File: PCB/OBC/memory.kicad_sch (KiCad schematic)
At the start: 14 parts, among them U10 TMUX1574PWR, U11 W25Q128JVSIQ, U12 TMUX1574PWR, U9 W25Q128JVSIQ

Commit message: Cambio de OCP
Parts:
- U10, U12: LCSC Part Name (none) -> C2673443
- U11, U9: LCSC Part Name (none) -> C97521

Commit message: Bom resistors
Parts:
- C53, C54, C56, C58: LCSC Part Name (none) -> C1711
- R16, R17, R18, R19: LCSC Part Name (none) -> C2907219
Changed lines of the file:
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@@
+			)
+		)
+		(property "LCSC Part Name" "C2907219"
+			(at 254 80.01 0)
+			(effects
+				(font
+					(size 1.27 1.27)
+				)
+				(hide yes)
 			)
 		)
@@
 		)
 		(property "Mouser" ""
+			(at 129.54 72.39 0)
+			(effects
+				(font
+					(size 1.27 1.27)
+				)
+				(hide yes)
+			)
+		)
+		(property "LCSC Part Name" "C1711"
 			(at 129.54 72.39 0)
 			(effects
@@
 			)
 		)
+		(property "LCSC Part Name" "C1711"
+			(at 269.24 127 0)
+			(effects
+				(font
+					(size 1.27 1.27)
+				)
+				(hide yes)
+			)
+		)
 		(pin "2"
 		)
@@
 			)
 		)
+		(property "LCSC Part Name" "C1711"
+			(at 199.39 62.23 0)
+			(effects
+				(font
+					(size 1.27 1.27)
+				)
+				(hide yes)
+			)
+		)
 		(pin "1"
 		)
@@
 			)
 		)
+		(property "LCSC Part Name" "C2907219"
+			(at 34.29 74.93 90)
+			(effects
+				(font
+					(size 1.27 1.27)
+				)
+				(hide yes)
+			)
+		)
 		(pin "2"
 		)
@@
 			)
 		)
+		(property "LCSC Part Name" "C2907219"
+			(at 109.22 67.31 0)
+			(effects
+				(font
+					(size 1.27 1.27)
+				)
+				(hide yes)
+			)
+		)
 		(pin "1"
 		)
@@
 			)
 		)
+		(property "LCSC Part Name" "C1711"
+			(at 119.38 116.84 0)
+			(effects
+				(font
+					(size 1.27 1.27)
+				)
+				(hide yes)
+			)
+		)
 		(pin "2"
 		)
@@
 			(at 173.99 88.9 90)
 			(effects
+				(font
+					(size 1.27 1.27)
+				)
+				(hide yes)
+			)
+		)
+		(property "LCSC Part Name" "C2907219"
+			(at 173.99 88.9 90)
+			(effects

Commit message: BOM terminado
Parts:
- C53, C54, C56, C58, U10, U11, U12, U9: now left out of the parts list
- C55: footprint XTAL_NX3215SA_NDK:XTAL_NX3215SA_NDK -> Capacitor_SMD:C_0805_2012Metric_Pad1.18x1.45mm_HandSolder; LCSC Part Name (none) -> C28323; now left out of the parts list
- C57: footprint TMUX1574PWR:PWP16_2P31X2P46_TEX -> Capacitor_SMD:C_0805_2012Metric_Pad1.18x1.45mm_HandSolder; LCSC Part Name (none) -> C28323; now left out of the parts list
- R16, R17, R18, R19: footprint (none) -> Resistor_SMD:R_0805_2012Metric_Pad1.20x1.40mm_HandSolder; now left out of the parts list
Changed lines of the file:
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@@
 		(unit 1)
 		(exclude_from_sim no)
-		(in_bom yes)
+		(in_bom no)
 		(on_board yes)
 		(dnp no)
@@
 			)
 		)
-		(property "Footprint" ""
+		(property "Footprint" "Resistor_SMD:R_0805_2012Metric_Pad1.20x1.40mm_HandSolder"
 			(at 252.222 80.01 90)
 			(effects
@@
 		(unit 1)
 		(exclude_from_sim no)
-		(in_bom yes)
+		(in_bom no)
 		(on_board yes)
 		(dnp no)
@@
 			)
 		)
-		(property "Footprint" "TMUX1574PWR:PWP16_2P31X2P46_TEX"
+		(property "Footprint" "Capacitor_SMD:C_0805_2012Metric_Pad1.18x1.45mm_HandSolder"
 			(at 213.0552 66.04 0)
 			(effects
@@
 			)
 		)
+		(property "LCSC Part Name" "C28323"
+			(at 212.09 62.23 0)
+			(effects
+				(font
+					(size 1.27 1.27)
+				)
+				(hide yes)
+			)
+		)
 		(pin "1"
 		)
@@
 		(unit 1)
 		(exclude_from_sim no)
-		(in_bom yes)
+		(in_bom no)
 		(on_board yes)
 		(dnp no)
@@
 			)
 		)
-		(property "Footprint" "XTAL_NX3215SA_NDK:XTAL_NX3215SA_NDK"
+		(property "Footprint" "Capacitor_SMD:C_0805_2012Metric_Pad1.18x1.45mm_HandSolder"
 			(at 143.2052 76.2 0)
 			(effects
@@
 			)
 		)
+		(property "LCSC Part Name" "C28323"
+			(at 142.24 72.39 0)
+			(effects
+				(font
+					(size 1.27 1.27)
+				)
+				(hide yes)
+			)
+		)
 		(pin "1"
 		)
@@
 		(unit 1)
 		(exclude_from_sim no)
-		(in_bom yes)
+		(in_bom no)
 		(on_board yes)
 		(dnp no)
@@
 		(unit 1)
 		(exclude_from_sim no)
-		(in_bom yes)
+		(in_bom no)
 		(on_board yes)
 		(dnp no)
@@
 		(unit 1)
 		(exclude_from_sim no)
-		(in_bom yes)
+		(in_bom no)
 		(on_board yes)
 		(dnp no)
@@
 		(unit 1)
 		(exclude_from_sim no)
-		(in_bom yes)
+		(in_bom no)
 		(on_board yes)
 		(dnp no)
@@
 		(unit 1)
 		(exclude_from_sim no)
-		(in_bom yes)
+		(in_bom no)
 		(on_board yes)
 		(dnp no)
@@
 			)
 		)
-		(property "Footprint" ""
+		(property "Footprint" "Resistor_SMD:R_0805_2012Metric_Pad1.20x1.40mm_HandSolder"
 			(at 34.29 73.152 90)
 			(effects
@@
 		(unit 1)
 		(exclude_from_sim no)
-		(in_bom yes)
+		(in_bom no)
 		(on_board yes)
 		(dnp no)
@@
 			)
 		)
-		(property "Footprint" ""
+		(property "Footprint" "Resistor_SMD:R_0805_2012Metric_Pad1.20x1.40mm_HandSolder"
 			(at 107.442 67.31 90)
 			(effects
@@
 		(unit 1)
 		(exclude_from_sim no)
-		(in_bom yes)
+		(in_bom no)
 		(on_board yes)
 		(dnp no)
@@
 		(unit 1)
 		(exclude_from_sim no)
-		(in_bom yes)
+		(in_bom no)
 		(on_board yes)
 		(dnp no)
@@
 		(unit 1)
 		(exclude_from_sim no)
-		(in_bom yes)
+		(in_bom no)
 		(on_board yes)
 		(dnp no)
@@
 			)
 		)
-		(property "Footprint" ""
+		(property "Footprint" "Resistor_SMD:R_0805_2012Metric_Pad1.20x1.40mm_HandSolder"
 			(at 173.99 87.122 90)
 			(effects
@@
 		(unit 1)
 		(exclude_from_sim no)
-		(in_bom yes)
+		(in_bom no)
 		(on_board yes)
 		(dnp no)
@@
 		(unit 1)
 		(exclude_from_sim no)
-		(in_bom yes)
+		(in_bom no)
 		(on_board yes)
 		(dnp no)

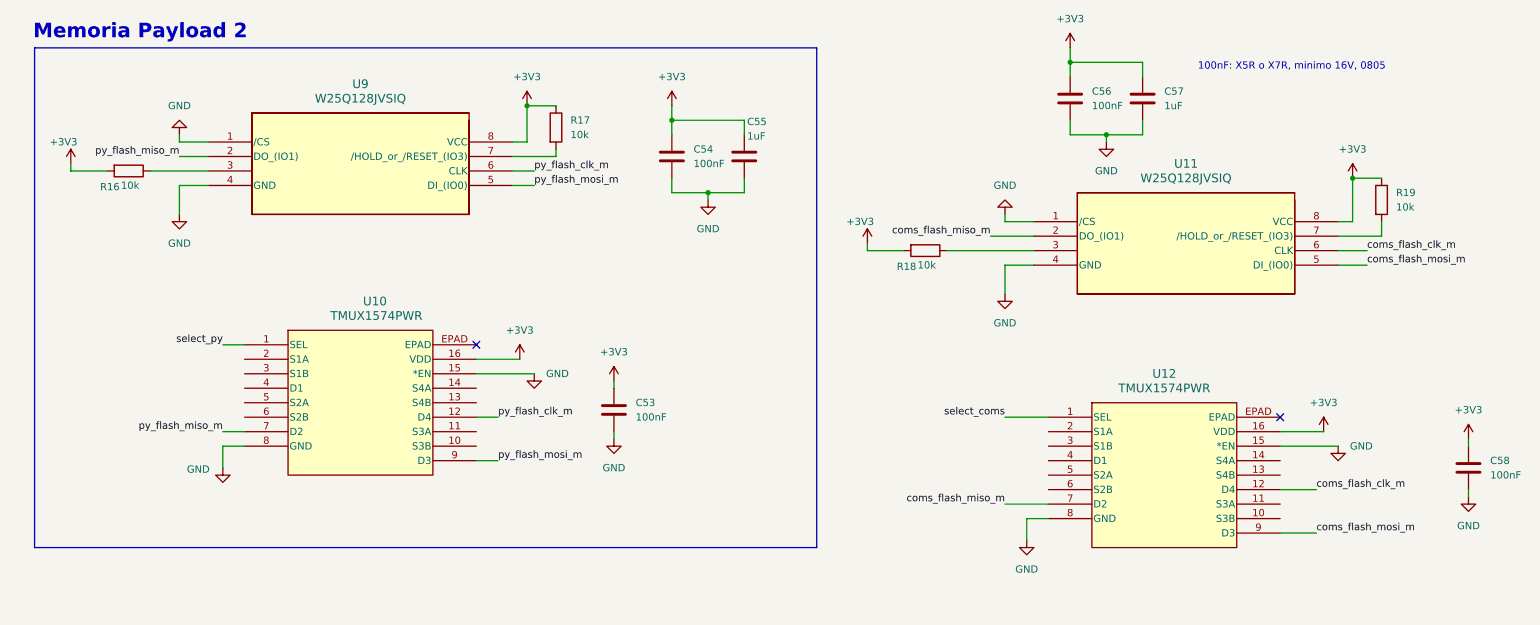
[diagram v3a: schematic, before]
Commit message: fix Tmux
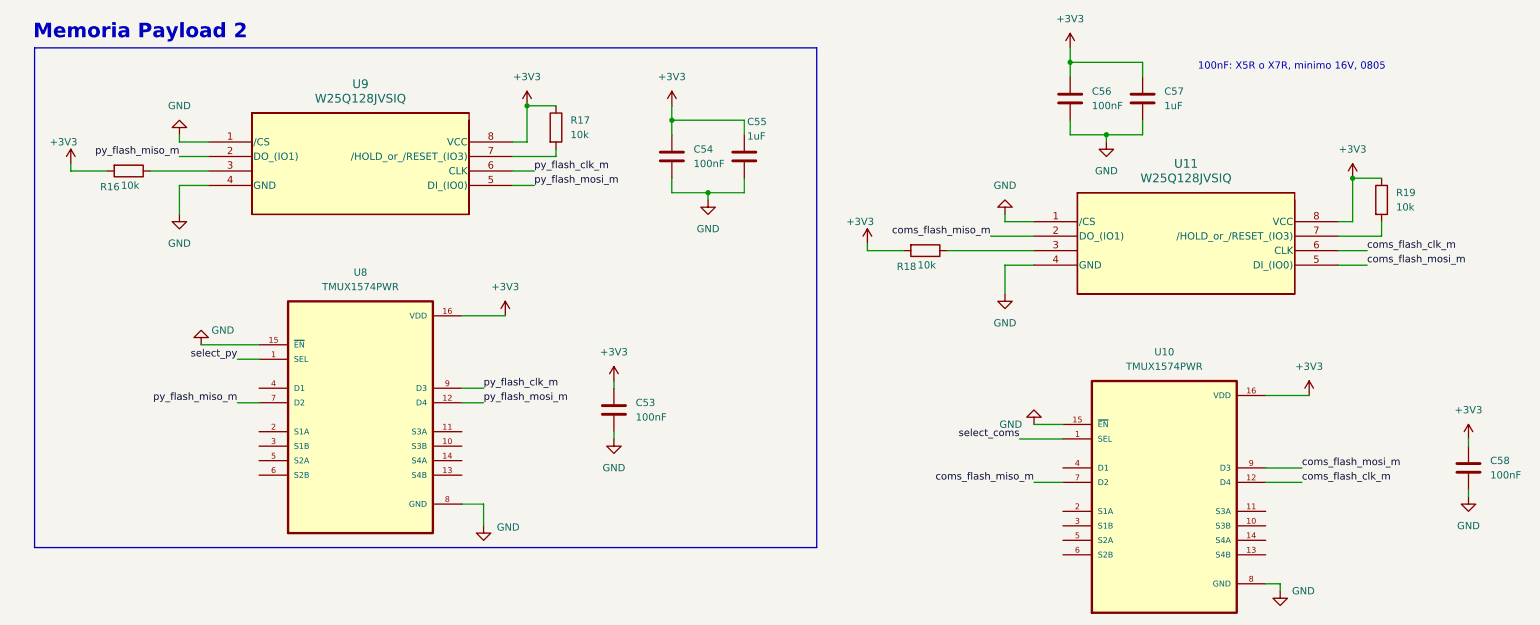
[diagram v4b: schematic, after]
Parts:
- removed U12: TMUX1574PWR, TMUX1574PWR:PWP16_2P31X2P46_TEX, symbol TMUX1574PWR:TMUX1574PWR
- added U8: TMUX1574PWR, TMUX1574PWR:SOP65P640X120-16N, symbol TMUX1574PWR:TMUX1574PWR
- C53, C54, C55, C56, C57, C58, R16, R17, R18, R19, U11, U9: now in the parts list
- U10: footprint TMUX1574PWR:PWP16_2P31X2P46_TEX -> TMUX1574PWR:SOP65P640X120-16N; LCSC Part Name C2673443 -> (none); now in the parts list
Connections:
- net +3V3: now also U8.16 (VDD)
- net GND: now also U8.15 (~{EN}), U8.8 (GND)
- net coms_flash_clk_m: now also U10.12 (D4)
- net coms_flash_miso_m: now also U10.7 (D2)
- net coms_flash_mosi_m: now also U10.9 (D3)
- net py_flash_clk_m: now also U8.9 (D3); no longer U10.12 (D4)
- net py_flash_miso_m: now also U8.7 (D2); no longer U10.7 (D2)
- net py_flash_mosi_m: now also U8.12 (D4); no longer U10.9 (D3)
- net select_coms: now also U10.1 (SEL)
- net select_py: now also U8.1 (SEL); no longer U10.1 (SEL)
- no-connect marks 2 -> 0
